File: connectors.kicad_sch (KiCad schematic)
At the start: 32 parts, among them J1 Conn_01x04, J10 Conn_02x02_Counter_Clockwise, J11 Conn_02x02_Counter_Clockwise, J12 Conn_02x02_Counter_Clockwise, J13 Conn_02x02_Counter_Clockwise, J14 Conn_02x02_Counter_Clockwise, J15 Conn_01x02, J16 Conn_01x02, J17 Conn_01x02, J18 Conn_01x02, J19 Conn_01x01, J20 Conn_01x01, J21 Conn_01x01, J22 Conn_01x01, J23 Conn_01x02, J24 Conn_01x02, J25 Conn_01x08, J26 Conn_01x08, J27 Conn_01x04, J3 Conn_01x04, J5 Conn_01x04, J7 Conn_02x02_Counter_Clockwise, J8 Conn_02x02_Counter_Clockwise, J9 Conn_02x02_Counter_Clockwise, P1 USB_C_Plug_USB2.0

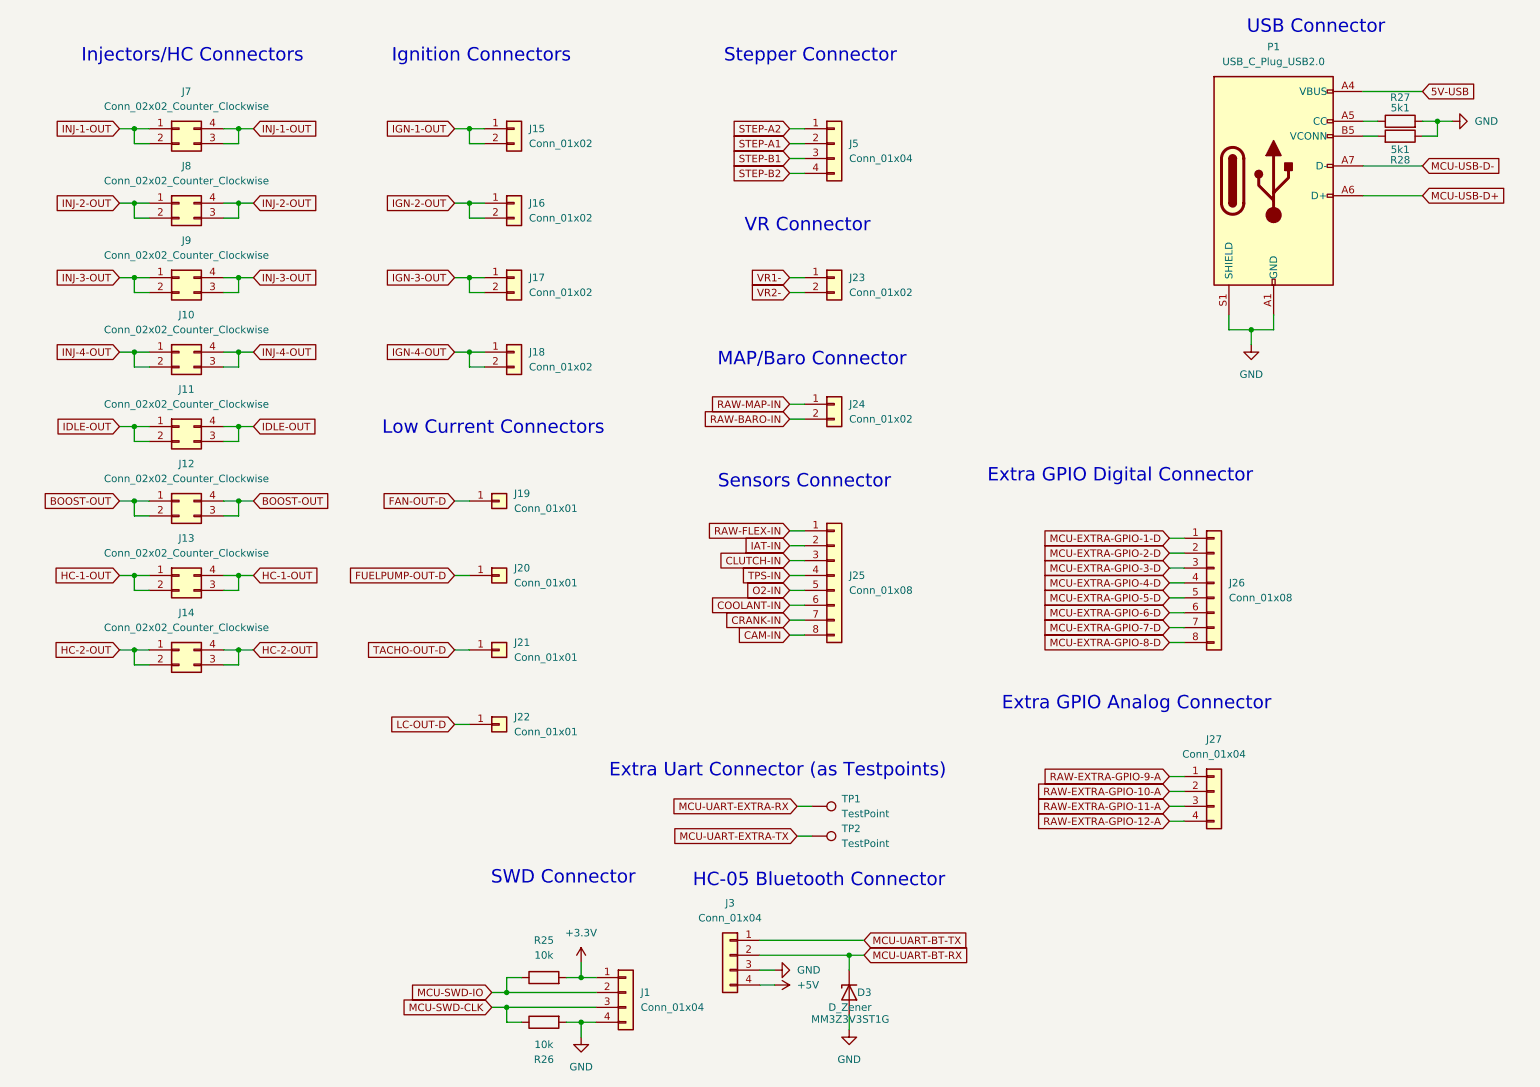
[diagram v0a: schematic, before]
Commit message: Fully connect all components
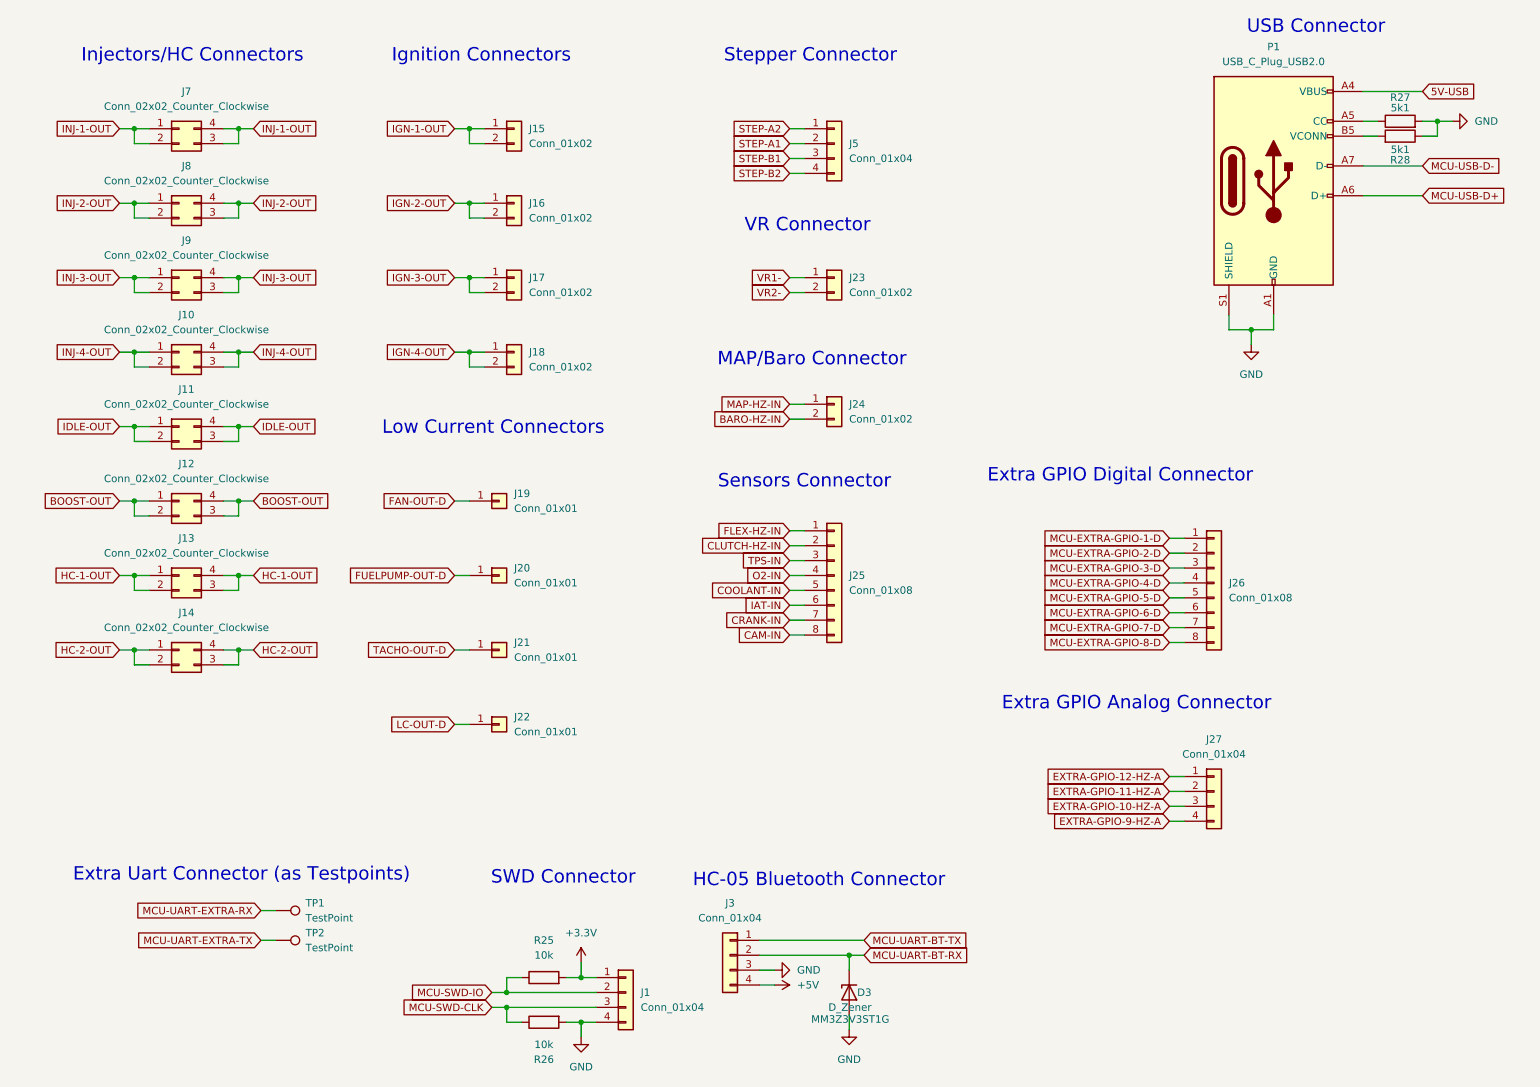
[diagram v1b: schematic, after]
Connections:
- net CLUTCH-IN is gone; now on net TPS-IN: J25.3 (Pin_3)
- net COOLANT-IN: now also J25.5 (Pin_5); no longer J25.6 (Pin_6)
- net IAT-IN: now also J25.6 (Pin_6); no longer J25.2 (Pin_2)
- net O2-IN: now also J25.4 (Pin_4); no longer J25.5 (Pin_5)
- net TPS-IN: no longer J25.4 (Pin_4)
- net RAW-BARO-IN renamed BARO-HZ-IN
- net RAW-EXTRA-GPIO-10-A renamed EXTRA-GPIO-11-HZ-A
- net RAW-EXTRA-GPIO-11-A renamed EXTRA-GPIO-10-HZ-A
- net RAW-EXTRA-GPIO-12-A renamed EXTRA-GPIO-9-HZ-A
- net RAW-EXTRA-GPIO-9-A renamed EXTRA-GPIO-12-HZ-A
- net RAW-FLEX-IN renamed FLEX-HZ-IN
- net RAW-MAP-IN renamed MAP-HZ-IN
- new net CLUTCH-HZ-IN: J25.2 (Pin_2)
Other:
- moved on the sheet: TP1, TP2
